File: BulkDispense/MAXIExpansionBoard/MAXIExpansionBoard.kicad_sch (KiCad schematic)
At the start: 25 parts, among them J1 BS1~4, J10 FS3, J11 R6~R7, J12 R8~R9, J13 OS1~4, J14 WV1~2, J15 FS2, J16 FS4, J17 Analog Inputs, J18 Digital IN + R0~R4, J19 Digital Outputs, J2 MV1~4, J20 R4~R9, J21 Flow Sensors, J3 WB/WL, J4 PS/PCV, J5 Screw_Terminal_01x02, J6 R0~R1, J7 R2~R3, J8 R4~R5, J9 FS1

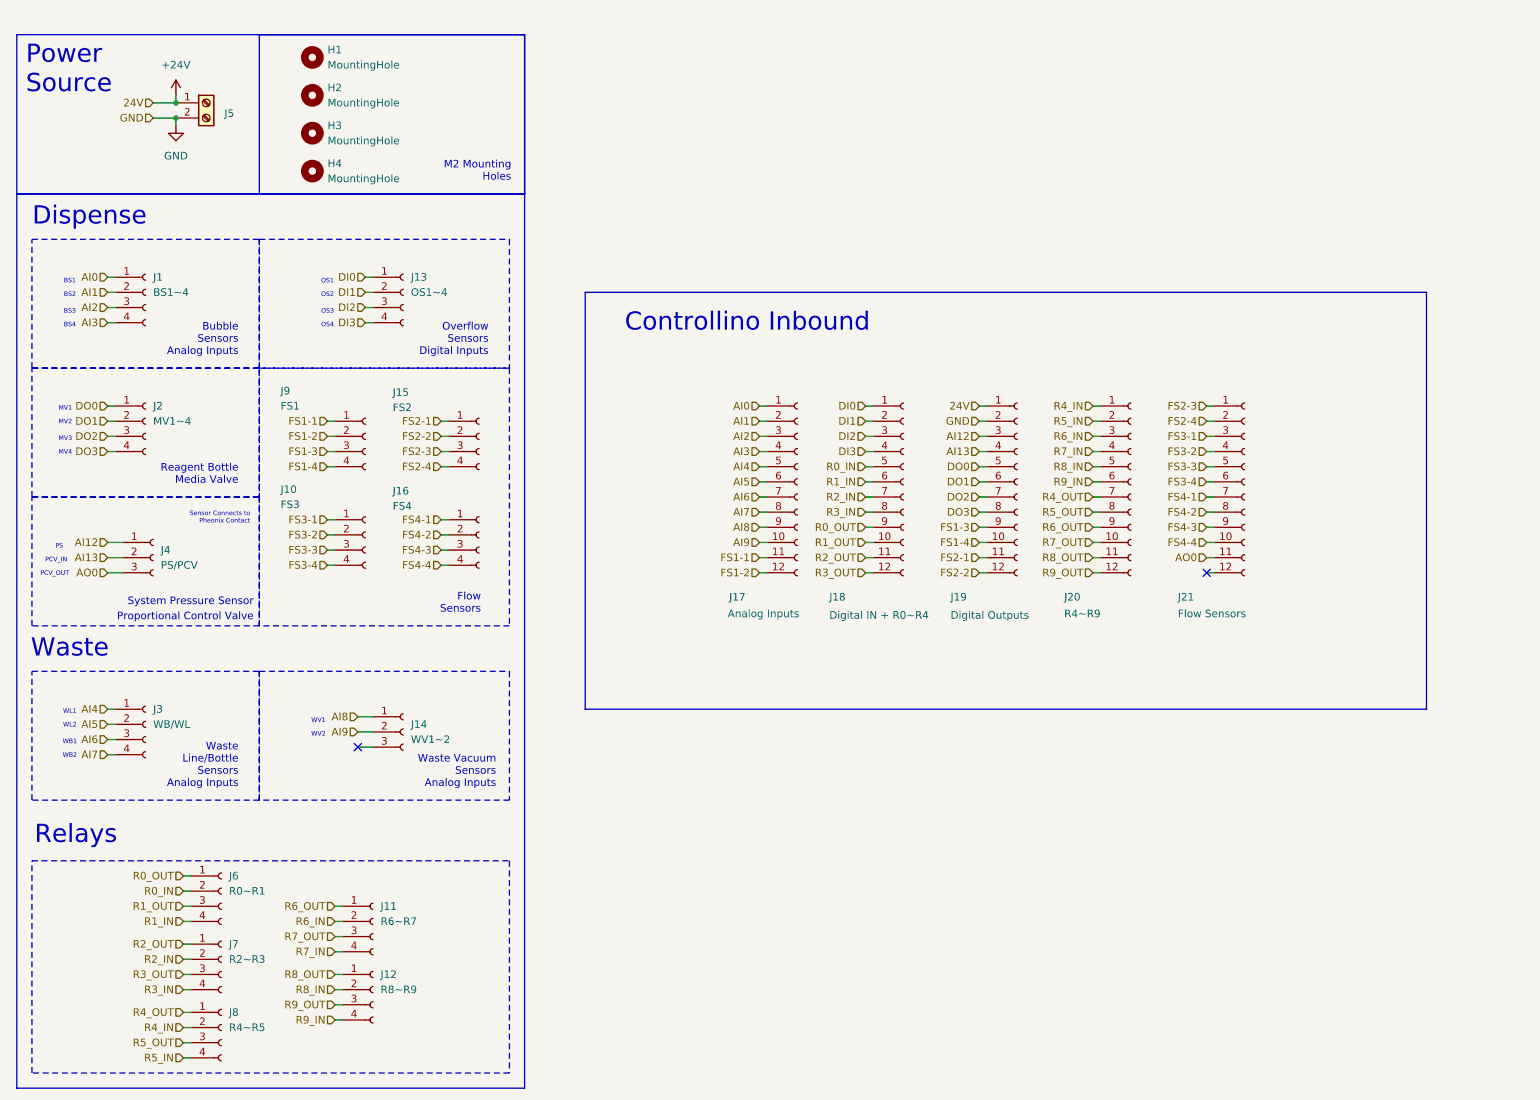
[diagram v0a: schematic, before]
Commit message: Design Overhaul
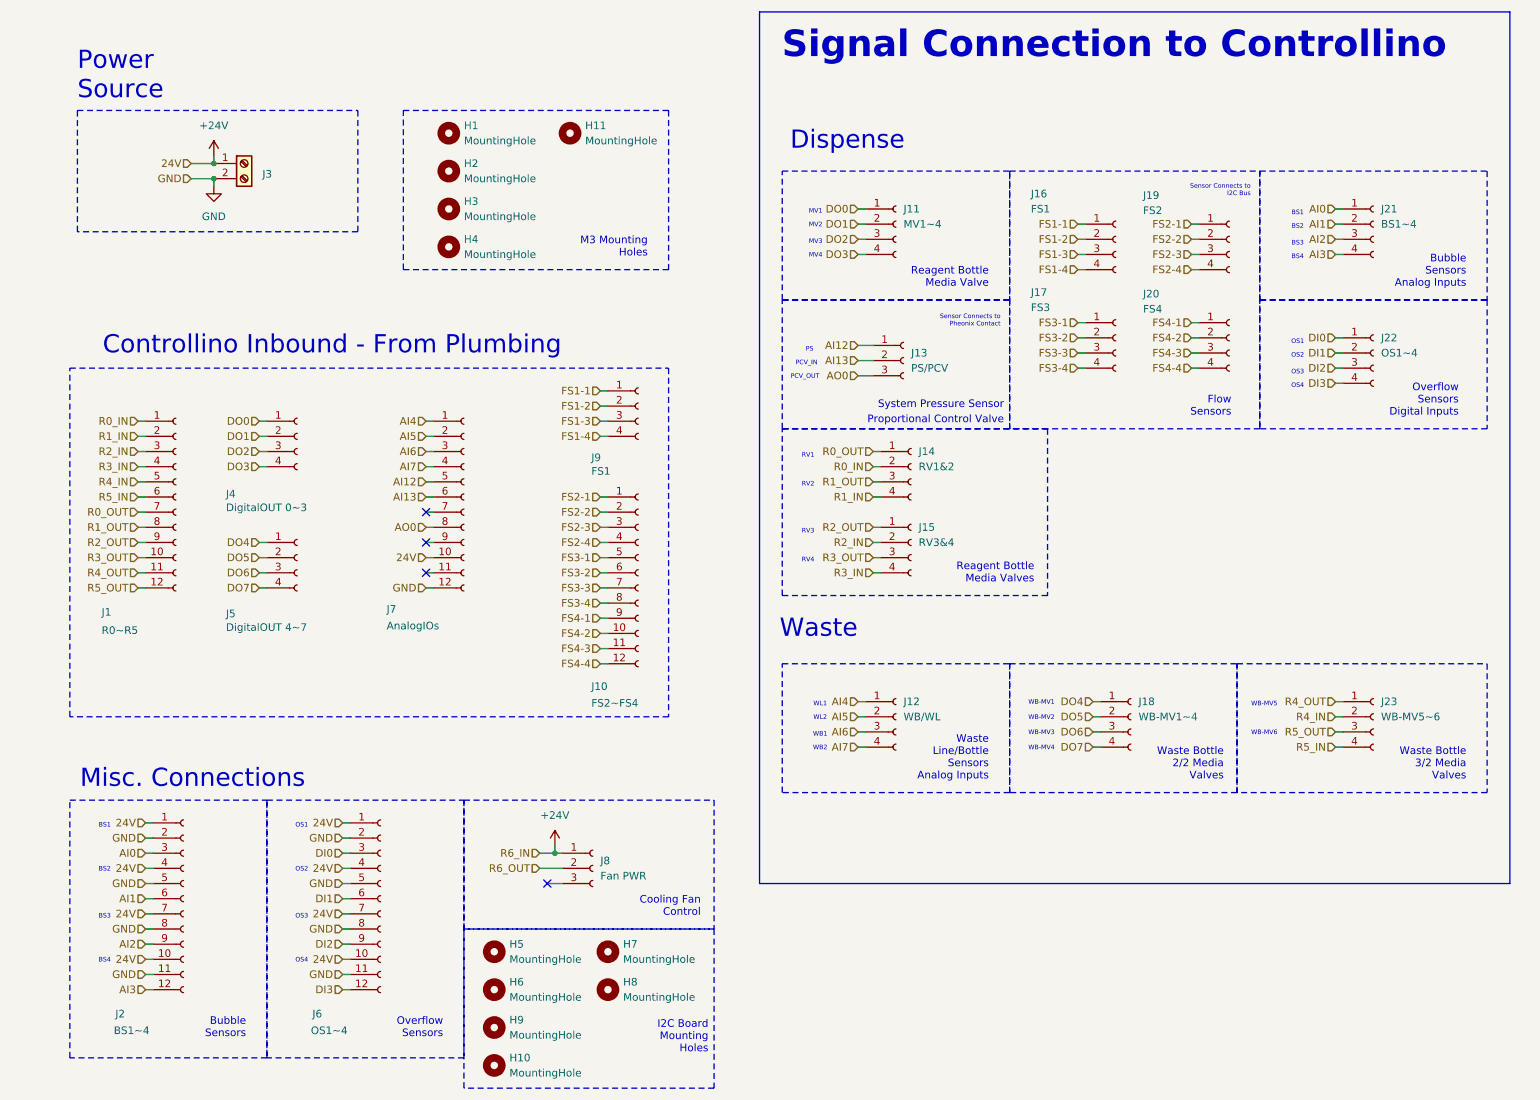
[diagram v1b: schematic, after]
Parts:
- removed J1: BS1~4, PartsLibrary:CONN_37204-62A3-004PL_3MM, symbol Connector:Conn_01x04_Socket
- removed J10: FS3, PartsLibrary:CONN_37204-62A3-004PL_3MM, symbol Connector:Conn_01x04_Socket
- removed J13: OS1~4, PartsLibrary:CONN_37204-62A3-004PL_3MM, symbol Connector:Conn_01x04_Socket
- removed J14: WV1~2, PartsLibrary:3720362A3003PL, symbol Connector:Conn_01x03_Socket
- removed J17: Analog Inputs, PartsLibrary:CONN_37212-62M3-003PL_3MM, symbol Connector:Conn_01x12_Socket
- removed J19: Digital Outputs, PartsLibrary:CONN_37212-62M3-003PL_3MM, symbol Connector:Conn_01x12_Socket
- removed J2: MV1~4, PartsLibrary:CONN_37204-62A3-004PL_3MM, symbol Connector:Conn_01x04_Socket
- removed J3: WB/WL, PartsLibrary:CONN_37204-62A3-004PL_3MM, symbol Connector:Conn_01x04_Socket
- removed J4: PS/PCV, PartsLibrary:3720362A3003PL, symbol Connector:Conn_01x03_Socket
- removed J5: Screw_Terminal_01x02, PartsLibrary:691137710002, symbol Connector:Screw_Terminal_01x02
- removed J6: R0~R1, PartsLibrary:CONN_37204-62A3-004PL_3MM, symbol Connector:Conn_01x04_Socket
- removed J7: R2~R3, PartsLibrary:CONN_37204-62A3-004PL_3MM, symbol Connector:Conn_01x04_Socket
- removed J8: R4~R5, PartsLibrary:CONN_37204-62A3-004PL_3MM, symbol Connector:Conn_01x04_Socket
- added H10, H5, H6, H7, H8, H9: MountingHole, MountingHole:MountingHole_2.5mm, symbol Mechanical:MountingHole
- added H11: MountingHole, MountingHole:MountingHole_3.2mm_M3, symbol Mechanical:MountingHole
- added J13: PS/PCV, PartsLibrary:3720362A3003PL, symbol Connector:Conn_01x03_Socket
- added J14: RV1&2, PartsLibrary:CONN_37204-62A3-004PL_3MM, symbol Connector:Conn_01x04_Socket
- added J17: FS3, PartsLibrary:CONN_37204-62A3-004PL_3MM, symbol Connector:Conn_01x04_Socket
- added J18: WB-MV1~4, PartsLibrary:CONN_37204-62A3-004PL_3MM, symbol Connector:Conn_01x04_Socket
- added J19: FS2, PartsLibrary:CONN_37204-62A3-004PL_3MM, symbol Connector:Conn_01x04_Socket
- added J2: BS1~4, PartsLibrary:CONN_37212-62M3-003PL_3MM, symbol Connector:Conn_01x12_Socket
- added J20: FS4, PartsLibrary:CONN_37204-62A3-004PL_3MM, symbol Connector:Conn_01x04_Socket
- added J21: BS1~4, PartsLibrary:CONN_37204-62A3-004PL_3MM, symbol Connector:Conn_01x04_Socket
- added J22: OS1~4, PartsLibrary:CONN_37204-62A3-004PL_3MM, symbol Connector:Conn_01x04_Socket
- added J23: WB-MV5~6, PartsLibrary:CONN_37204-62A3-004PL_3MM, symbol Connector:Conn_01x04_Socket
- added J3: Screw_Terminal_01x02, PartsLibrary:691137710002, symbol Connector:Screw_Terminal_01x02
- added J4: DigitalOUT 0~3, PartsLibrary:CONN_37204-62A3-004PL_3MM, symbol Connector:Conn_01x04_Socket
- added J5: DigitalOUT 4~7, PartsLibrary:CONN_37204-62A3-004PL_3MM, symbol Connector:Conn_01x04_Socket
- added J6: OS1~4, PartsLibrary:CONN_37212-62M3-003PL_3MM, symbol Connector:Conn_01x12_Socket
- added J8: Fan PWR, PartsLibrary:3720362A3003PL, symbol Connector:Conn_01x03_Socket
- H1, H2, H3, H4: footprint MountingHole:MountingHole_2.2mm_M2 -> MountingHole:MountingHole_3.2mm_M3
- J1: renamed from J18; value Digital IN + R0~R4 -> R0~R5
- J10: renamed from J21; value Flow Sensors -> FS2~FS4
- J11: value R6~R7 -> MV1~4
- J12: value R8~R9 -> WB/WL
- J15: value FS2 -> RV3&4
- J16: value FS4 -> FS1
- J7: renamed from J20; value R4~R9 -> AnalogIOs
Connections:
- net +24V: now also J7.10 (Pin_10), J2.1 (Pin_1), J2.10 (Pin_10), J2.4 (Pin_4), J2.7 (Pin_7), J3.1 (Pin_1), J6.1 (Pin_1), J6.10 (Pin_10), J6.4 (Pin_4), J6.7 (Pin_7), J8.1 (Pin_1)
- net AI0: now also J2.3 (Pin_3), J21.1 (Pin_1)
- net AI1: now also J2.6 (Pin_6), J21.2 (Pin_2)
- net AI12: now also J7.5 (Pin_5), J13.1 (Pin_1)
- net AI13: now also J7.6 (Pin_6), J13.2 (Pin_2)
- net AI2: now also J2.9 (Pin_9), J21.3 (Pin_3)
- net AI3: now also J2.12 (Pin_12), J21.4 (Pin_4)
- net AI4: now also J12.1 (Pin_1), J7.1 (Pin_1)
- net AI5: now also J12.2 (Pin_2), J7.2 (Pin_2)
- net AI6: now also J12.3 (Pin_3), J7.3 (Pin_3)
- net AI7: now also J12.4 (Pin_4), J7.4 (Pin_4)
- net AO0: now also J7.8 (Pin_8), J13.3 (Pin_3); no longer J10.11 (Pin_11)
- net DI0: now also J22.1 (Pin_1), J6.3 (Pin_3); no longer J1.1 (Pin_1)
- net DI1: now also J22.2 (Pin_2), J6.6 (Pin_6); no longer J1.2 (Pin_2)
- net DI2: now also J22.3 (Pin_3), J6.9 (Pin_9); no longer J1.3 (Pin_3)
- net DI3: now also J22.4 (Pin_4), J6.12 (Pin_12); no longer J1.4 (Pin_4)
- net DO0: now also J11.1 (Pin_1), J4.1 (Pin_1)
- net DO1: now also J11.2 (Pin_2), J4.2 (Pin_2)
- net DO2: now also J11.3 (Pin_3), J4.3 (Pin_3)
- net DO3: now also J11.4 (Pin_4), J4.4 (Pin_4)
- net FS1-1: now also J16.1 (Pin_1)
- net FS1-2: now also J16.2 (Pin_2)
- net FS1-3: now also J16.3 (Pin_3)
- net FS1-4: now also J16.4 (Pin_4)
- net FS2-1: now also J10.1 (Pin_1), J19.1 (Pin_1); no longer J15.1 (Pin_1)
- net FS2-2: now also J10.2 (Pin_2), J19.2 (Pin_2); no longer J15.2 (Pin_2)
- net FS2-3: now also J10.3 (Pin_3), J19.3 (Pin_3); no longer J10.1 (Pin_1), J15.3 (Pin_3)
- net FS2-4: now also J10.4 (Pin_4), J19.4 (Pin_4); no longer J10.2 (Pin_2), J15.4 (Pin_4)
- net FS3-1: now also J10.5 (Pin_5), J17.1 (Pin_1); no longer J10.3 (Pin_3)
- net FS3-2: now also J10.6 (Pin_6), J17.2 (Pin_2); no longer J10.4 (Pin_4)
- net FS3-3: now also J10.7 (Pin_7), J17.3 (Pin_3); no longer J10.5 (Pin_5)
- net FS3-4: now also J10.8 (Pin_8), J17.4 (Pin_4); no longer J10.6 (Pin_6)
- net FS4-1: now also J10.9 (Pin_9), J20.1 (Pin_1); no longer J10.7 (Pin_7), J16.1 (Pin_1)
- net FS4-2: now also J10.10 (Pin_10), J20.2 (Pin_2); no longer J10.8 (Pin_8), J16.2 (Pin_2)
- net FS4-3: now also J10.11 (Pin_11), J20.3 (Pin_3); no longer J10.9 (Pin_9), J16.3 (Pin_3)
- net FS4-4: now also J10.12 (Pin_12), J20.4 (Pin_4); no longer J10.10 (Pin_10), J16.4 (Pin_4)
- net GND: now also J7.12 (Pin_12), J2.11 (Pin_11), J2.2 (Pin_2), J2.5 (Pin_5), J2.8 (Pin_8), J3.2 (Pin_2), J6.11 (Pin_11), J6.2 (Pin_2), J6.5 (Pin_5), J6.8 (Pin_8)
- net R0_IN: now also J1.1 (Pin_1), J14.2 (Pin_2); no longer J1.5 (Pin_5)
- net R0_OUT: now also J1.7 (Pin_7), J14.1 (Pin_1); no longer J1.9 (Pin_9)
- net R1_IN: now also J1.2 (Pin_2), J14.4 (Pin_4); no longer J1.6 (Pin_6)
- net R1_OUT: now also J1.8 (Pin_8), J14.3 (Pin_3); no longer J1.10 (Pin_10)
- net R2_IN: now also J1.3 (Pin_3), J15.2 (Pin_2); no longer J1.7 (Pin_7)
- net R2_OUT: now also J1.9 (Pin_9), J15.1 (Pin_1); no longer J1.11 (Pin_11)
- net R3_IN: now also J1.4 (Pin_4), J15.4 (Pin_4); no longer J1.8 (Pin_8)
- net R3_OUT: now also J1.10 (Pin_10), J15.3 (Pin_3); no longer J1.12 (Pin_12)
- net R4_IN: now also J1.5 (Pin_5), J23.2 (Pin_2); no longer J7.1 (Pin_1)
- net R4_OUT: now also J1.11 (Pin_11), J23.1 (Pin_1); no longer J7.7 (Pin_7)
- net R5_IN: now also J1.6 (Pin_6), J23.4 (Pin_4); no longer J7.2 (Pin_2)
- net R5_OUT: now also J1.12 (Pin_12), J23.3 (Pin_3); no longer J7.8 (Pin_8)
- net R6_OUT: now also J8.2 (Pin_2); no longer J11.1 (Pin_1), J7.9 (Pin_9)
- removed net R6_IN: J11.2 (Pin_2), J7.3 (Pin_3)
- removed net R7_IN: J11.4 (Pin_4), J7.4 (Pin_4)
- removed net R7_OUT: J11.3 (Pin_3), J7.10 (Pin_10)
- removed net R8_IN: J12.2 (Pin_2), J7.5 (Pin_5)
- net R8_OUT: no longer names the net of J7.11 (Pin_11)
- net R8_OUT: no longer J12.1 (Pin_1)
- removed net R9_IN: J12.4 (Pin_4), J7.6 (Pin_6)
- removed net R9_OUT: J12.3 (Pin_3), J7.12 (Pin_12)
- new net DO4: J18.1 (Pin_1), J5.1 (Pin_1)
- new net DO5: J18.2 (Pin_2), J5.2 (Pin_2)
- new net DO6: J18.3 (Pin_3), J5.3 (Pin_3)
- new net DO7: J18.4 (Pin_4), J5.4 (Pin_4)
- no-connect marks 2 -> 4
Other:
- note added: "Controllino Inbound - From Plumbing"
- note added: "Misc. Connections"
- note added: "RV1"
- note added: "RV2"
- note added: "RV3"
- note added: "RV4"
- note added: "Sensor Connects to I2C Bus"
- note added: "Signal Connection to Controllino"
- note added: "WB-MV1"
- note added: "WB-MV2"
- note added: "WB-MV3"
- note added: "WB-MV4"
- note added: "WB-MV5"
- note added: "WB-MV6"
- note removed: "Controllino Inbound"
- note removed: "Relays"
- note removed: "WV1"
- note removed: "WV2"
- moved on the sheet: J1, J10, J7
